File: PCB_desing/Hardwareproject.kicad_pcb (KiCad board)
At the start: 2 copper layers, 21 parts, among them J1 Barrel_Jack, J2 Conn_01x01, J3 Conn_01x01, J4 Barrel_Jack, Q1 IRF540N, T1 PA0184NL, U1 lt1246

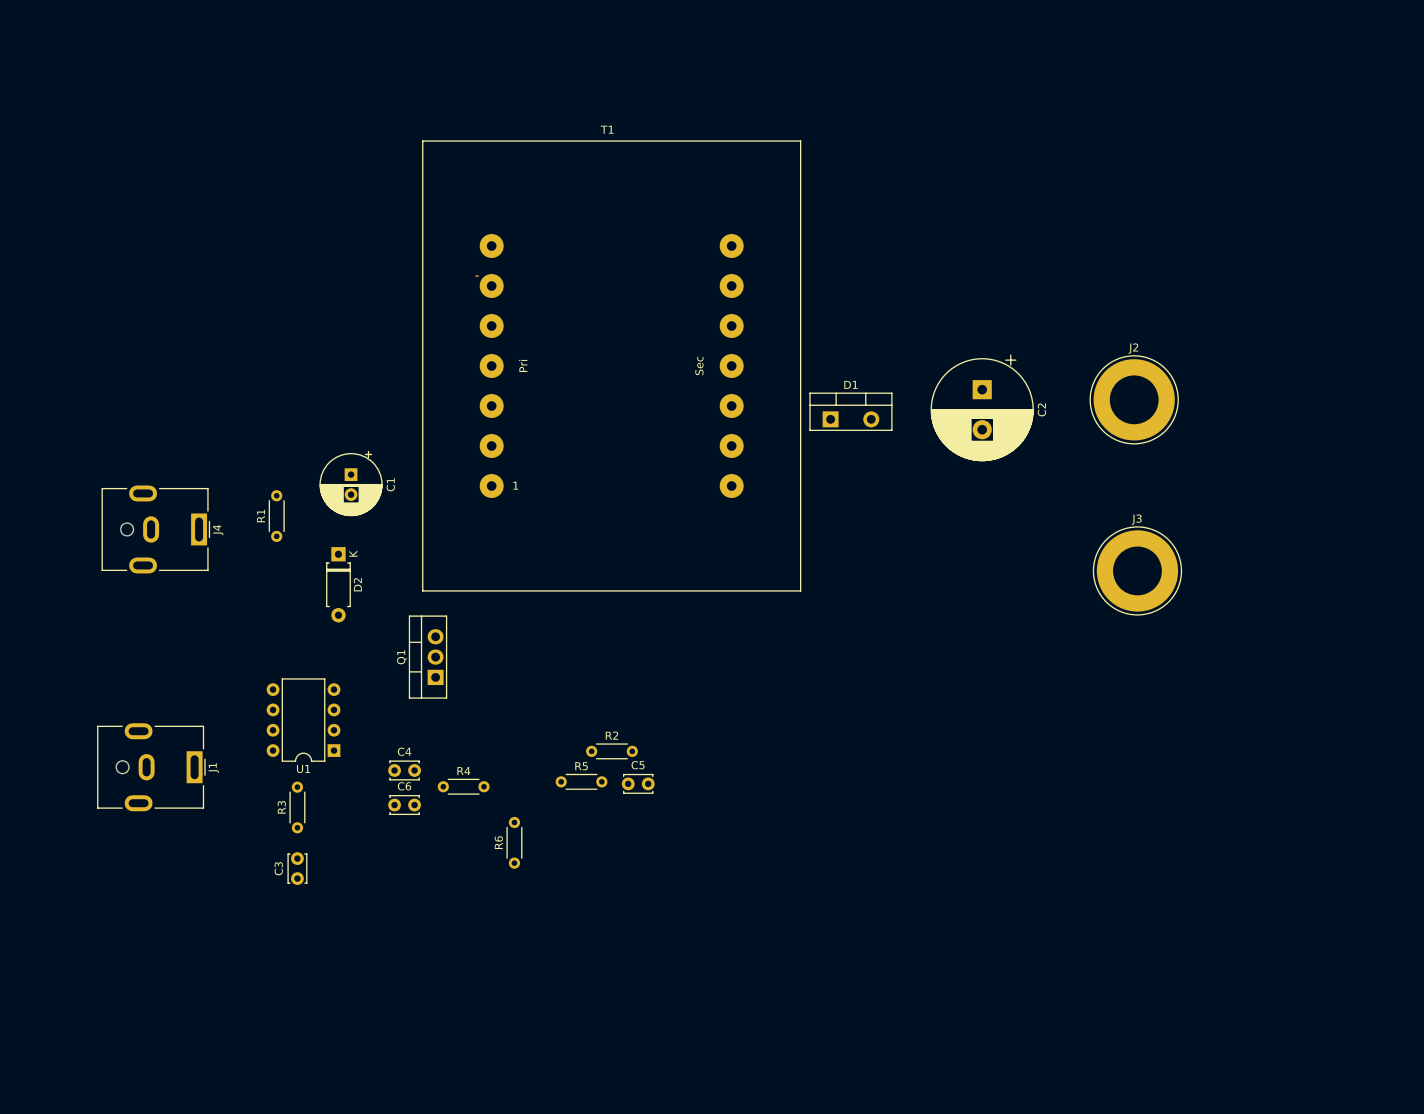
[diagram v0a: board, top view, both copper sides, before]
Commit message: Updates
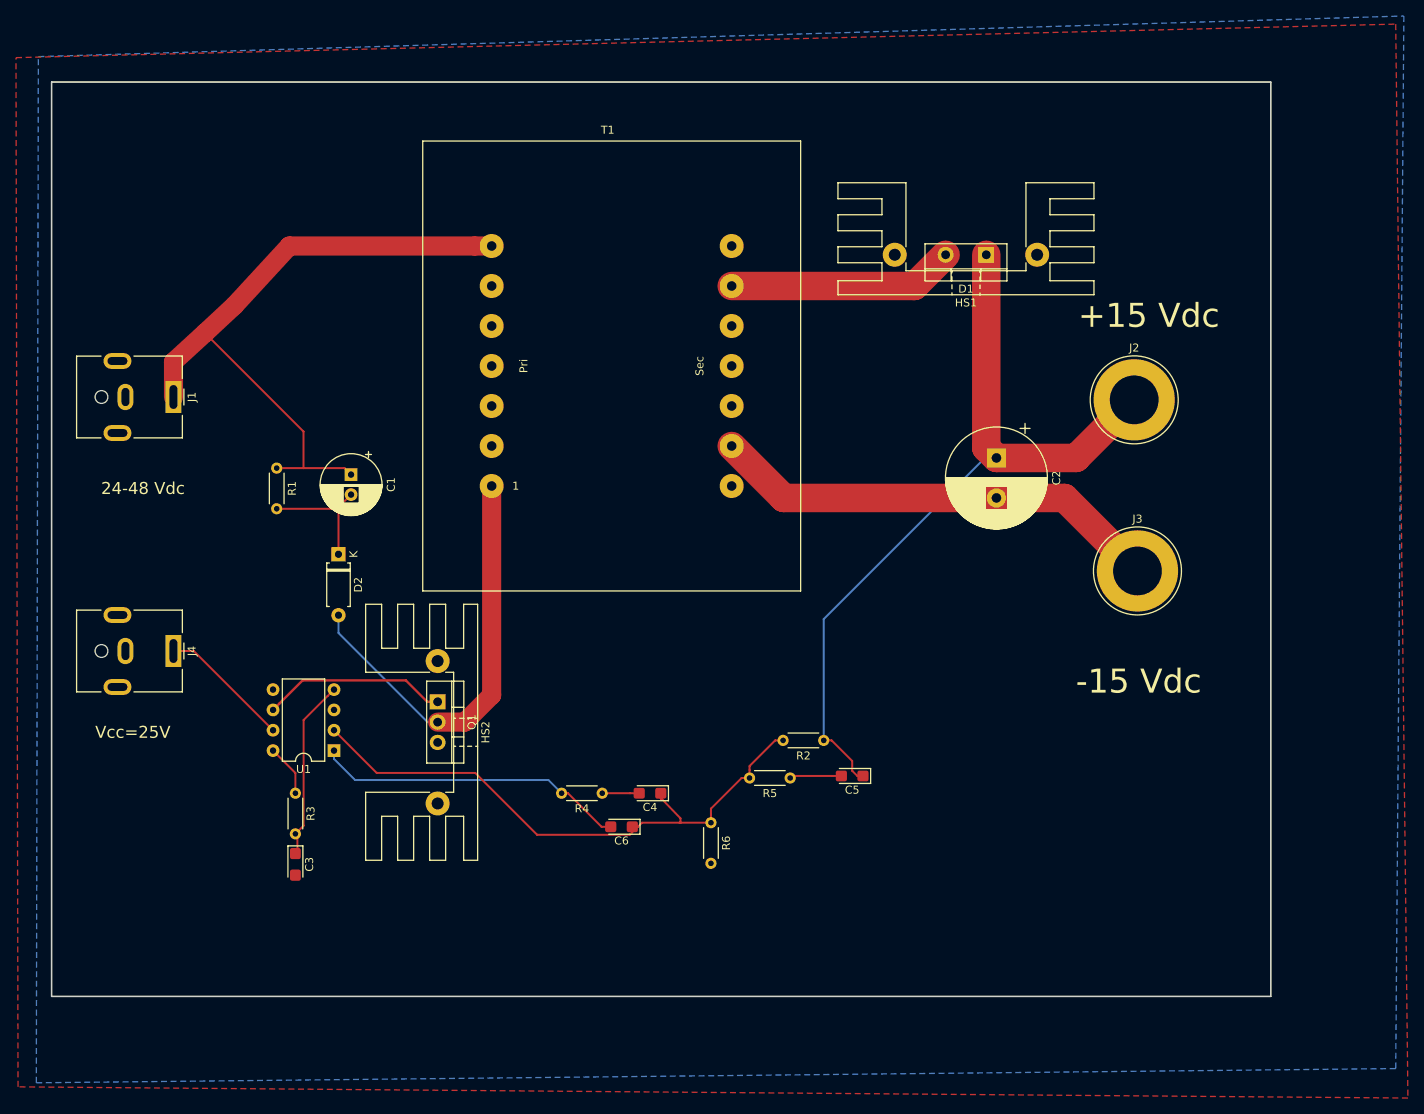
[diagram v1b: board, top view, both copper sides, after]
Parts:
- added HS1: Heatsink, Heatsink:Heatsink_Stonecold_HS-132_32x14mm_2xFixation1.5mm, F.Cu at (139.7, 47.0)
- added HS2: Heatsink, Heatsink:Heatsink_Stonecold_HS-132_32x14mm_2xFixation1.5mm, F.Cu at (73.7, 106.7)
- C3, C4, C5, C6: footprint Capacitor_THT:C_Disc_D3.4mm_W2.1mm_P2.50mm -> Capacitor_Tantalum_SMD:CP_EIA-3216-10_Kemet-I
- moved J1 46.4 mm to (40.6, 64.8)
- moved C4 32.1 mm to (100.2, 114.3), turned to 180 degrees
- moved R2 29.0 mm to (121.9, 107.7), turned to 180 degrees
- moved R5 28.6 mm to (117.7, 112.4), turned to 180 degrees
- moved C6 28.5 mm to (96.6, 118.5), turned to 180 degrees
- moved D1 28.3 mm to (142.2, 47.0), turned to 180 degrees
- moved C5 28.0 mm to (125.5, 112.1), turned to 180 degrees
- moved R6 25.1 mm to (107.8, 118.0), turned to 270 degrees
- moved R4 19.9 mm to (94.2, 114.3), turned to 180 degrees
- moved J4 15.5 mm to (40.6, 96.5)
- moved C2 8.72 mm to (143.5, 72.4)
- moved R1 8.53 mm to (53.5, 73.7), turned to 270 degrees
- moved R3 4.33 mm to (55.9, 114.3), turned to 270 degrees
- moved Q1 3.06 mm to (73.7, 102.9), turned to 270 degrees
- moved C3 1.80 mm to (55.9, 123.2), turned to 270 degrees
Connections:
- C2 pad 2: Net-(C2-Pad2) -> GND
- J3 pad 1: Net-(C2-Pad2) -> GND
- T1 pad 5: Net-(C2-Pad2) -> GND
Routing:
- net Net-(C2-Pad1): track 0.00 -> 100.3 mm
- net Net-(C1-Pad1): track 0.23 -> 81.8 mm
- net Net-(C4-Pad1): track 0.00 -> 73.5 mm
- net GND: track 0.00 -> 57.2 mm
- net Net-(D2-Pad2): track 0.00 -> 53.5 mm
- net Net-(C6-Pad2): track 0.00 -> 39.2 mm
- net Net-(D1-Pad2): track 0.00 -> 28.4 mm
- net Net-(Q1-Pad1): track 0.00 -> 23.2 mm
- net Net-(C3-Pad1): track 0.00 -> 22.7 mm
- net Net-(J4-Pad1): track 0.00 -> 16.5 mm
- net Net-(C1-Pad2): track 0.00 -> 15.9 mm
- net Net-(C5-Pad2): track 0.00 -> 6.50 mm
- net Net-(R3-Pad1): track 0.00 -> 6.49 mm
- net Net-(C4-Pad2): track 0.00 -> 4.62 mm
- added copper zone on B.Cu, net GND
- added copper zone on F.Cu, net GND
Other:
- board outline added: 152.4 x 114.3 mm
- board text added: "+15 Vdc"
- board text added: "-15 Vdc"
- board text added: "24-48 Vdc"
- board text added: "Vcc=25V"
